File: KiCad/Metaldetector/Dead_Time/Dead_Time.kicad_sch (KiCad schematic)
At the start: 18 parts, among them Q7 PNP_BC558, U1 L272M, U2 74AUC2G04

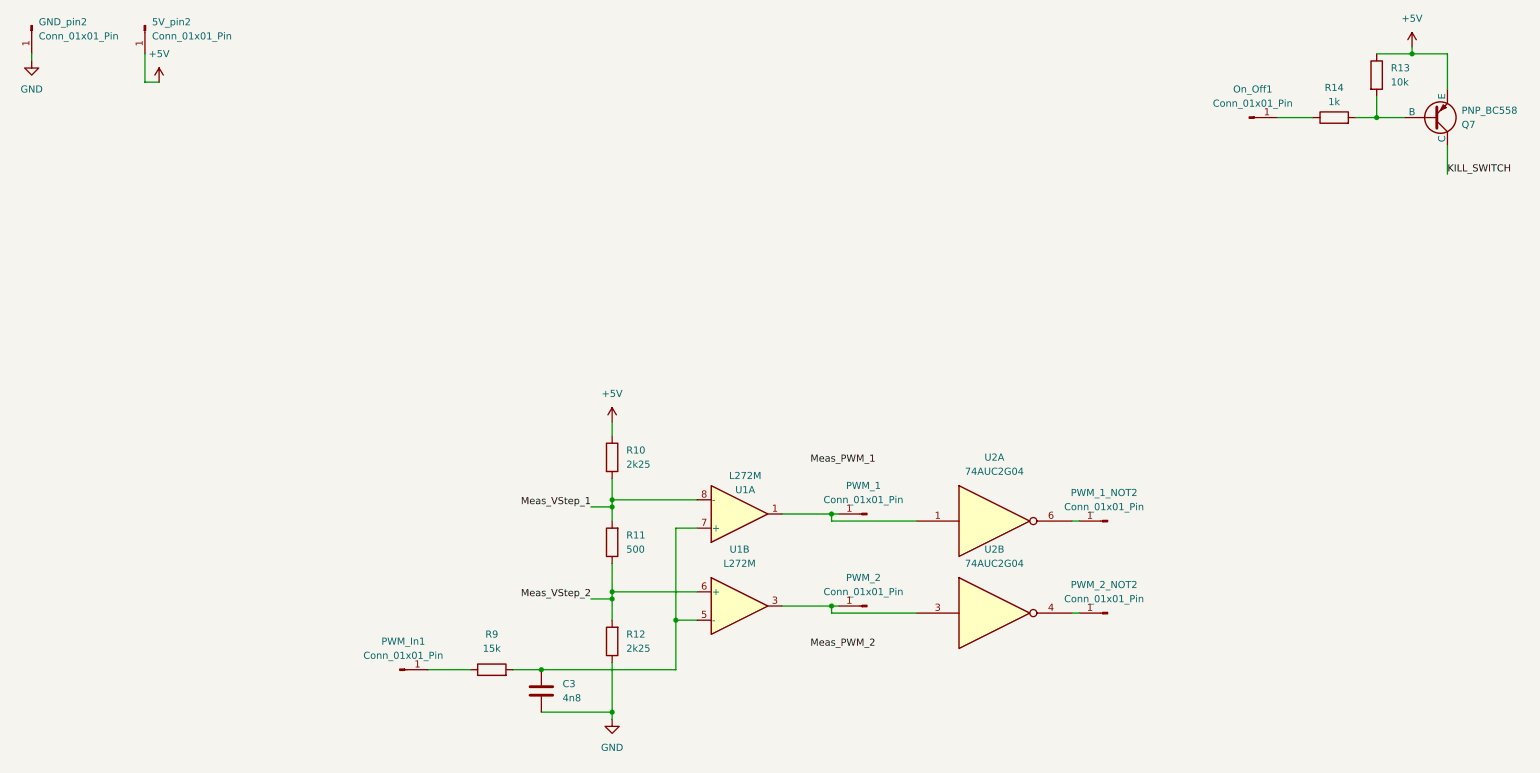
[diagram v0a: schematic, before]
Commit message: ændret kicad opsætning
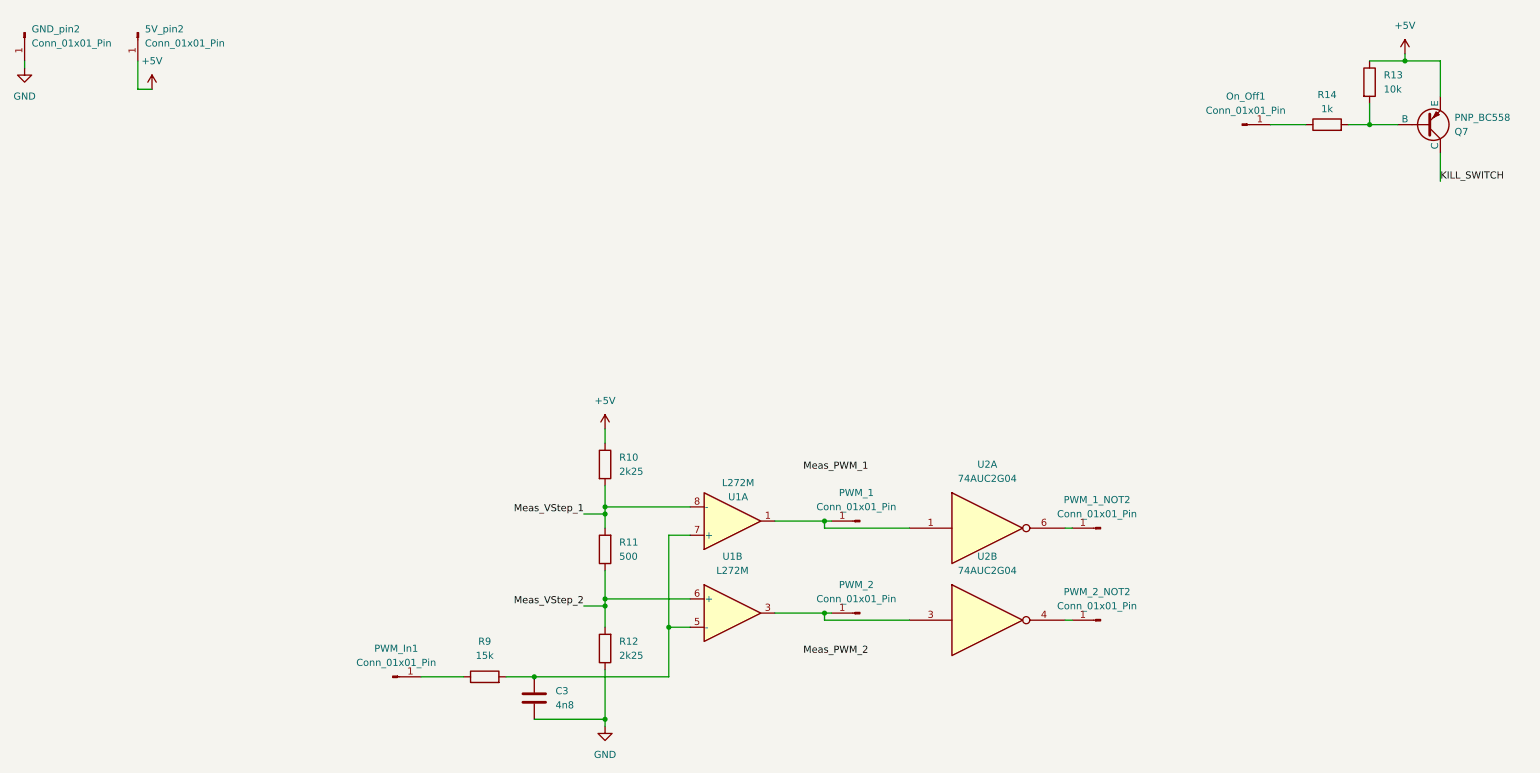
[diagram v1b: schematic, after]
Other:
- moved on the sheet: 5V_pin2, C3, GND_pin2, On_Off1, PWM_1, PWM_1_NOT2, PWM_2, PWM_2_NOT2, PWM_In1, Q7, R10, R11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
